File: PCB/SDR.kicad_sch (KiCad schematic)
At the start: 190 parts, among them IC1 RFSW6042TR7, IC2 RFSW6042TR7, IC5 CMX992Q3, J1 SMA, J11 SMA, J12 SMA, J13 Nucleo_GPIO, J14 SMA, J15 Nucleo_GPIO, J2 Nucleo_GPIO, J3 Nucleo_GPIO, J4 Nucleo_GPIO, J5 FPGA, J6 Tang Nano, J7 Tang Nano, J8 Tang Nano, J9 USB_C_Receptacle_PowerOnly_6P, U1 SGL0622Z, U10 ECS-45K15B, U2 ADF4351BCPZ-RL7, U3 ATX-H12-F-10.000MHZ-F25-T, U4 MASWSS0115, U6 LTC2323CUFD-12-PBF, U7 LT1762-2.5, U8 LT1962-3.3, U9 ECS-45K15B

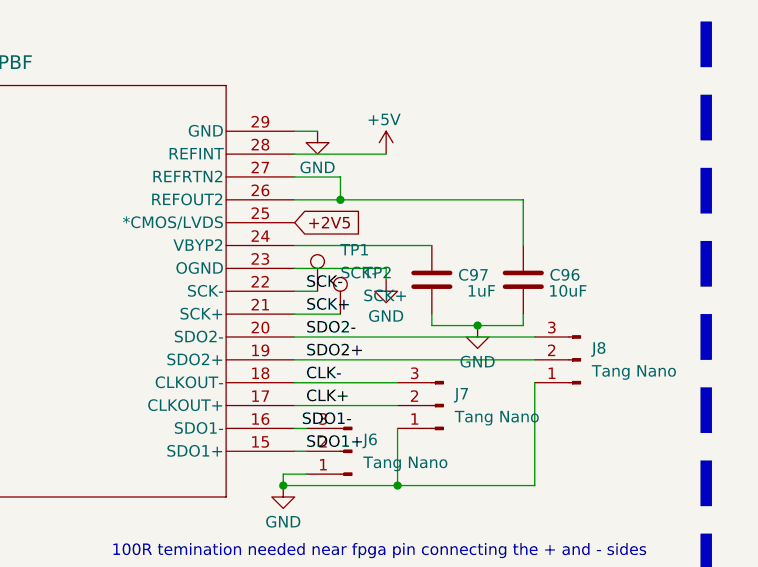
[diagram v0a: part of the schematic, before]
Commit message: Add files via upload
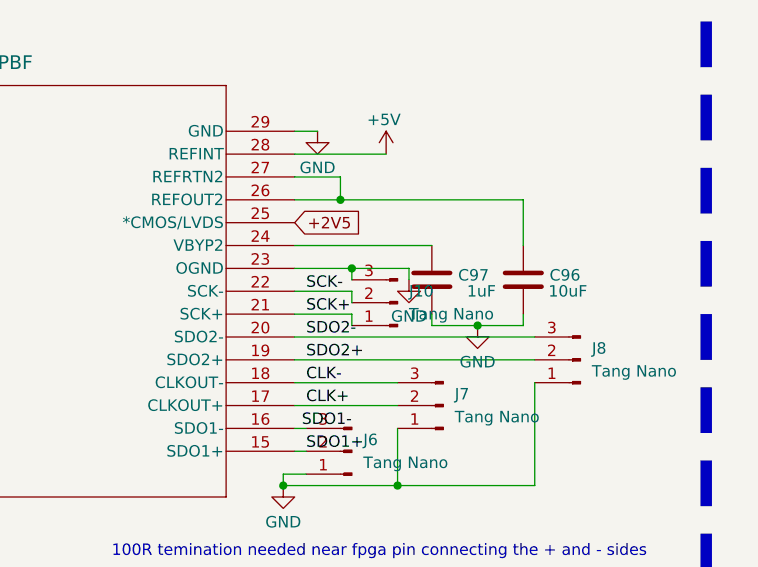
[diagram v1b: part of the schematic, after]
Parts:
- removed TP1: SCK-, TestPoint:TestPoint_Pad_D3.0mm, symbol Connector:TestPoint
- removed TP2: SCK+, TestPoint:TestPoint_Pad_D3.0mm, symbol Connector:TestPoint
- added J10: Tang Nano, Connector_Wire:SolderWire-0.25sqmm_1x03_P4.5mm_D0.65mm_OD2mm, symbol Connector:Conn_01x03_Pin
- D1: footprint LED_SMD:LED_0201_0603Metric -> LED_SMD:LED_0603_1608Metric
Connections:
- net GND: now also J10.3 (Pin_3)
- net SCK+: now also J10.1 (Pin_1)
- net SCK-: now also J10.2 (Pin_2)
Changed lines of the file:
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@@
 	)
 	(junction
+		(at 539.75 295.91)
+		(diameter 0)
+		(color 0 0 0 0)
+	)
+	(junction
 		(at 290.83 344.17)
 		(diameter 0)
@@
 	(wire
 		(pts
-			(xy 533.4 300.99) (xy 538.48 300.99)
+			(xy 533.4 300.99) (xy 539.75 300.99)
 		)
 		(stroke
@@
 	(wire
 		(pts
-			(xy 543.56 297.18) (xy 543.56 295.91)
+			(xy 546.1 297.18) (xy 546.1 295.91)
 		)
 		(stroke
@@
 	(wire
 		(pts
-			(xy 533.4 298.45) (xy 535.94 298.45)
+			(xy 533.4 298.45) (xy 539.75 298.45)
 		)
 		(stroke
@@
 	(wire
 		(pts
+			(xy 539.75 295.91) (xy 533.4 295.91)
+		)
+		(stroke
+			(width 0)
+			(type default)
+		)
+	)
+	(wire
+		(pts
 			(xy 490.22 140.97) (xy 492.76 140.97)
 		)
@@
 	(wire
 		(pts
+			(xy 539.75 295.91) (xy 539.75 297.18)
+		)
+		(stroke
+			(width 0)
+			(type default)
+		)
+	)
+	(wire
+		(pts
 			(xy 190.5 166.37) (xy 196.85 166.37)
 		)
@@
 	(wire
 		(pts
-			(xy 543.56 295.91) (xy 533.4 295.91)
+			(xy 546.1 295.91) (xy 539.75 295.91)
 		)
 		(stroke
@@
 	(wire
 		(pts
+			(xy 539.75 298.45) (xy 539.75 299.72)
+		)
+		(stroke
+			(width 0)
+			(type default)
+		)
+	)
+	(wire
+		(pts
 			(xy 111.76 304.8) (xy 114.3 304.8)
 		)
@@
 	(wire
 		(pts
+			(xy 539.75 300.99) (xy 539.75 302.26)
+		)
+		(stroke
+			(width 0)
+			(type default)
+		)
+	)
+	(wire
+		(pts
 			(xy 546.1 161.29) (xy 546.1 163.83)
 		)
@@
 			)
 		)
-		(property "Footprint" "LED_SMD:LED_0201_0603Metric"
+		(property "Footprint" "LED_SMD:LED_0603_1608Metric"
 			(at 162.56 281.94 0)
 			(hide yes)
@@
 	)
 	(symbol
-		(lib_id "Connector:TestPoint")
-		(at 538.48 300.99 0)
-		(unit 1)
-		(body_style 1)
-		(exclude_from_sim no)
-		(in_bom yes)
-		(on_board yes)
-		(in_pos_files yes)
-		(dnp no)
-		(fields_autoplaced yes)
-		(property "Reference" "TP2"
-			(at 541.02 296.4179 0)
-			(show_name no)
-			(do_not_autoplace no)
-			(effects
-				(font
-					(size 1.27 1.27)
-				)
-				(justify left)
-			)
-		)
-		(property "Value" "SCK+"
-			(at 541.02 298.9579 0)
-			(show_name no)
-			(do_not_autoplace no)
-			(effects
-				(font
-					(size 1.27 1.27)
-				)
-				(justify left)
-			)
-		)
-		(property "Footprint" "TestPoint:TestPoint_Pad_D3.0mm"
-			(at 543.56 300.99 0)
-			(hide yes)
-			(show_name no)
-			(do_not_autoplace no)
-			(effects
-				(font
-					(size 1.27 1.27)
-				)
-			)
-		)
-		(property "Datasheet" ""
-			(at 543.56 300.99 0)
-			(hide yes)
-			(show_name no)
-			(do_not_autoplace no)
-			(effects
-				(font
-					(size 1.27 1.27)
-				)
-			)
-		)
-		(property "Description" "test point"
-			(at 538.48 300.99 0)
-			(hide yes)
-			(show_name no)
-			(do_not_autoplace no)
-			(effects
-				(font
-					(size 1.27 1.27)
-				)
-			)
-		)
-		(pin "1"
-		)
-		(instances
-			(project "SDR"
-				(path "/8d810f61-405f-4958-b618-c99ce9e26cf2"
-					(reference "TP2")
-					(unit 1)
-				)
-			)
-		)
-	)
-	(symbol
 		(lib_id "Device:L")
 		(at 180.34 166.37 90)
@@
 	(symbol
 		(lib_id "power:GND")
-		(at 543.56 297.18 0)
+		(at 546.1 297.18 0)
 		(unit 1)
 		(body_style 1)
@@
 		(dnp no)
 		(property "Reference" "#PWR072"
-			(at 543.56 303.53 0)
+			(at 546.1 303.53 0)
 			(hide yes)
 			(show_name no)
@@
 		)
 		(property "Value" "GND"
-			(at 543.56 301.244 0)
+			(at 546.1 301.244 0)
 			(show_name no)
 			(do_not_autoplace no)
@@
 		)
 		(property "Footprint" ""
-			(at 543.56 297.18 0)
+			(at 546.1 297.18 0)
 			(hide yes)
 			(show_name no)
@@
 		)
 		(property "Datasheet" ""
-			(at 543.56 297.18 0)
+			(at 546.1 297.18 0)
 			(hide yes)
 			(show_name no)
@@
 		)
 		(property "Description" "Power symbol creates a global label with name \"GND\" , ground"
-			(at 543.56 297.18 0)
+			(at 546.1 297.18 0)
 			(hide yes)
 			(show_name no)
@@
 	)
 	(symbol
-		(lib_id "Connector:TestPoint")
-		(at 535.94 298.45 0)
-		(unit 1)
-		(body_style 1)
-		(exclude_from_sim no)
-		(in_bom yes)
-		(on_board yes)
-		(in_pos_files yes)
-		(dnp no)
-		(property "Reference" "TP1"
-			(at 538.48 293.8779 0)
-			(show_name no)
-			(do_not_autoplace no)
-			(effects
-				(font
-					(size 1.27 1.27)
-				)
-				(justify left)
-			)
-		)
-		(property "Value" "SCK-"
-			(at 538.48 296.4179 0)
-			(show_name no)
-			(do_not_autoplace no)
-			(effects
-				(font
-					(size 1.27 1.27)
-				)
-				(justify left)
-			)
-		)
-		(property "Footprint" "TestPoint:TestPoint_Pad_D3.0mm"
-			(at 541.02 298.45 0)
-			(hide yes)
-			(show_name no)
-			(do_not_autoplace no)
-			(effects
-				(font
-					(size 1.27 1.27)
-				)
-			)
-		)
-		(property "Datasheet" ""
-			(at 541.02 298.45 0)
-			(hide yes)
-			(show_name no)
-			(do_not_autoplace no)
-			(effects
-				(font
-					(size 1.27 1.27)
-				)
-			)
-		)
-		(property "Description" "test point"
-			(at 535.94 298.45 0)
-			(hide yes)
-			(show_name no)
-			(do_not_autoplace no)
-			(effects
-				(font
-					(size 1.27 1.27)
-				)
-			)
-		)
-		(pin "1"
-		)
-		(instances
-			(project "SDR"
-				(path "/8d810f61-405f-4958-b618-c99ce9e26cf2"
-					(reference "TP1")
-					(unit 1)
-				)
-			)
-		)
-	)
-	(symbol
 		(lib_id "Device:R")
 		(at 353.06 247.65 90)
@@
 					(unit 1)
 				)
+			)
+		)
+	)
+	(symbol
+		(lib_id "Connector:Conn_01x03_Pin")
+		(at 544.83 299.72 180)
+		(unit 1)
+		(body_style 1)
+		(exclude_from_sim no)
+		(in_bom yes)
+		(on_board yes)
+		(in_pos_files yes)
+		(dnp no)
+		(fields_autoplaced yes)
+		(property "Reference" "J10"
+			(at 546.1 298.4499 0)
+			(show_name no)
+			(do_not_autoplace no)
+			(effects
+				(font
+					(size 1.27 1.27)
+				)
+				(justify right)
+			)
+		)
+		(property "Value" "Tang Nano"
+			(at 546.1 300.9899 0)
+			(show_name no)
+			(do_not_autoplace no)
+			(effects
+				(font
+					(size 1.27 1.27)
+				)
+				(justify right)
+			)
+		)
+		(property "Footprint" "Connector_Wire:SolderWire-0.25sqmm_1x03_P4.5mm_D0.65mm_OD2mm"
+			(at 544.83 299.72 0)
+			(hide yes)
+			(show_name no)
+			(do_not_autoplace no)
+			(effects
+				(font
+					(size 1.27 1.27)
+				)
+			)
+		)
+		(property "Datasheet" ""
+			(at 544.83 299.72 0)
+			(hide yes)
+			(show_name no)
+			(do_not_autoplace no)
+			(effects
+				(font
+					(size 1.27 1.27)
+				)
+			)
+		)
+		(property "Description" "Generic connector, single row, 01x03, script generated"
+			(at 544.83 299.72 0)
+			(hide yes)
+			(show_name no)
+			(do_not_autoplace no)
+			(effects
+				(font
+					(size 1.27 1.27)
+				)
+			)
+		)
+		(pin "2"
+		)
+		(pin "1"
+		)
+		(pin "3"
+		)
+		(instances
+			(project "SDR"
+				(path "/8d810f61-405f-4958-b618-c99ce9e26cf2"
+					(reference "J10")
+					(unit 1)
+				)
